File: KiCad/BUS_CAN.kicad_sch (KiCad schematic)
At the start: 5 parts, among them J2 DE9_Pins_MountingHoles, U4 SN65HVD230

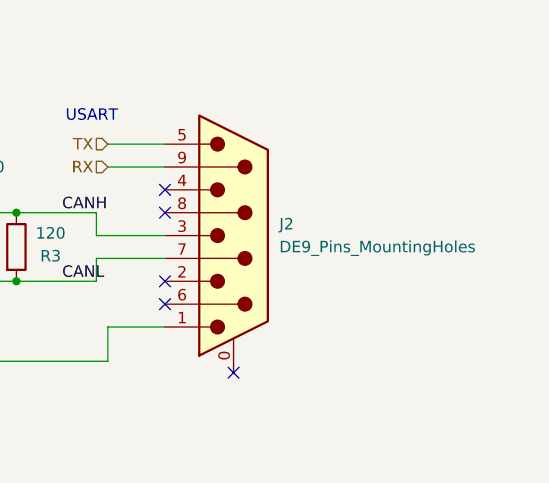
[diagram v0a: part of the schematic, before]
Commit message: 1ra versióPCB
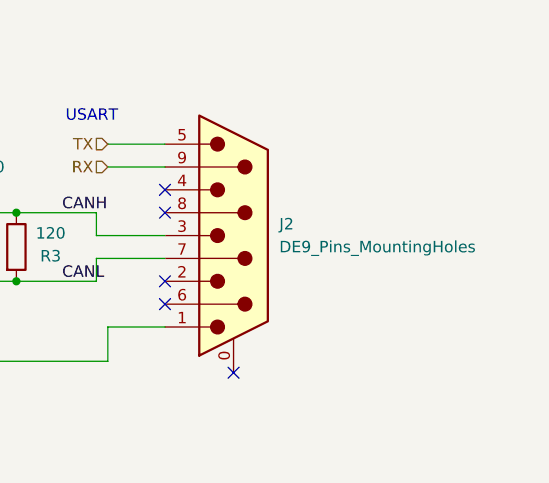
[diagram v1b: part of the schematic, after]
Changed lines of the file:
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@@
 		(on_board yes)
 		(dnp no)
-		(fields_autoplaced yes)
 		(property "Reference" "J2"
 			(at 186.69 88.8999 0)
@@
 		)
 		(property "Value" "DE9_Pins_MountingHoles"
-			(at 186.69 91.4399 0)
+			(at 186.69 91.44 0)
 			(effects
 				(font
